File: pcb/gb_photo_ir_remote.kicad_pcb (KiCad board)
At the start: 2 copper layers, 28 x 41 mm, 10 parts, among them SW1 SW_Push_SPDT, SW2 SW_Push_SPDT, U1 NE555P

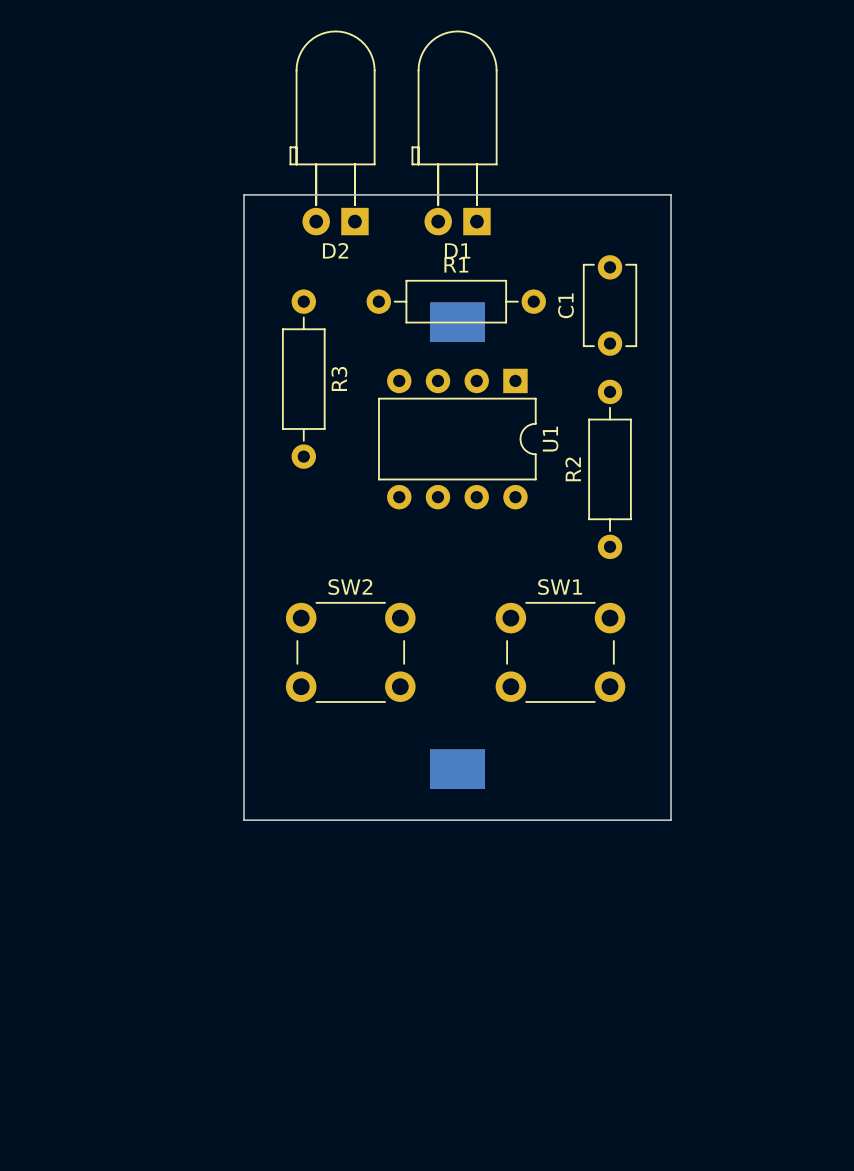
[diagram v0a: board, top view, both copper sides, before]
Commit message: build
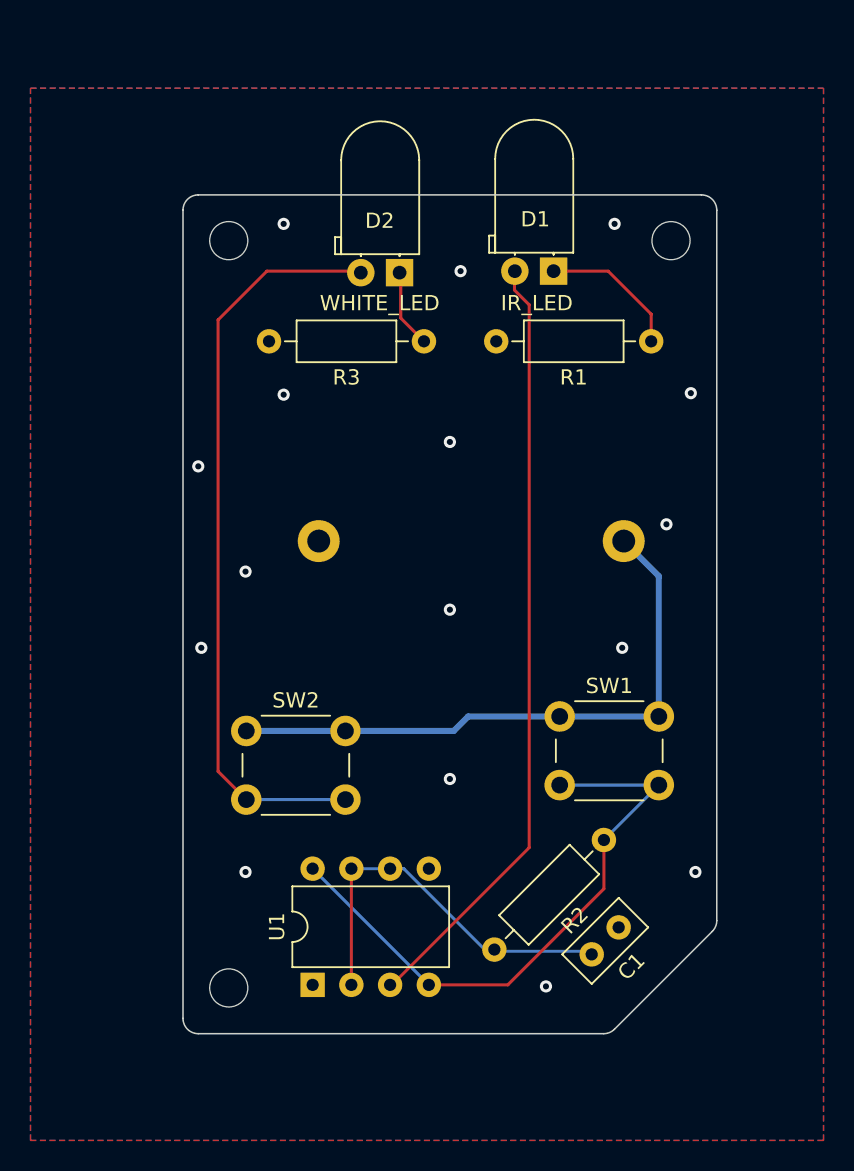
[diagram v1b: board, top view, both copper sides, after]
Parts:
- added M1: MountingHole_2.5mm, MountingHole:MountingHole_2.5mm, F.Cu at (123.0, 31.0)
- added M2: MountingHole_2.5mm, MountingHole:MountingHole_2.5mm, F.Cu at (152.0, 31.0)
- added M3: MountingHole_2.5mm, MountingHole:MountingHole_2.5mm, F.Cu at (123.0, 80.0)
- BT1: footprint Battery:BatteryHolder_Keystone_1060_1x2032 -> REB:REB_BatteryHolder_2032
- C1: footprint Capacitor_THT:C_Disc_D5.1mm_W3.2mm_P5.00mm -> Capacitor_THT:C_Disc_D5.0mm_W2.5mm_P2.50mm
- D1, D2: footprint LED_THT:LED_D5.0mm_Horizontal_O3.81mm_Z3.0mm -> LED_THT:LED_D5.0mm_Horizontal_O1.27mm_Z3.0mm
- moved U1 41.8 mm to (128.5, 79.8), turned to 90 degrees
- moved C1 40.1 mm to (146.8, 77.8), turned to 45 degrees
- moved R2 19.2 mm to (147.6, 70.3), turned to -135 degrees
- moved R1 18.0 mm to (150.7, 37.6), turned to 180 degrees
- moved R3 8.30 mm to (135.8, 37.6), turned to 180 degrees
- moved SW2 8.23 mm to (124.2, 63.1)
- moved SW1 7.20 mm to (144.7, 62.2)
- moved D1 5.98 mm to (144.3, 33.0)
- moved D2 4.45 mm to (134.2, 33.1)
- moved BT1 1.24 mm to (136.8, 50.7), turned to 0 degrees
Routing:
- net /OUT: track 0.00 -> 51.1 mm
- net Net-(D2-A): track 0.00 -> 49.4 mm
- net +BATT: track 0.00 -> 39.9 mm
- net /VIN: track 0.00 -> 39.7 mm
- net /DIS: track 0.00 -> 25.7 mm
- net Net-(D1-K): track 0.00 -> 9.38 mm
- net Net-(D2-K): track 0.00 -> 5.16 mm
- net GND: vias 0 -> 16
- added copper zone on B.Cu, net GND
- added copper zone on F.Cu, net GND
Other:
- board size 28 x 41 mm -> 35 x 55 mm
